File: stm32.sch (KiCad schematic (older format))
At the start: 33 parts, among them P1 USB_OTG, P2 CONN_01X04, U3 STM32F407VETx, U4 USBLC6-4SC6, Y2 25M, Y3 RTC

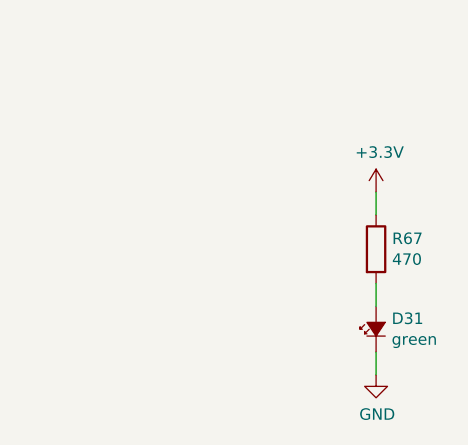
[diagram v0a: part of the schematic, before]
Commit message: eth phy
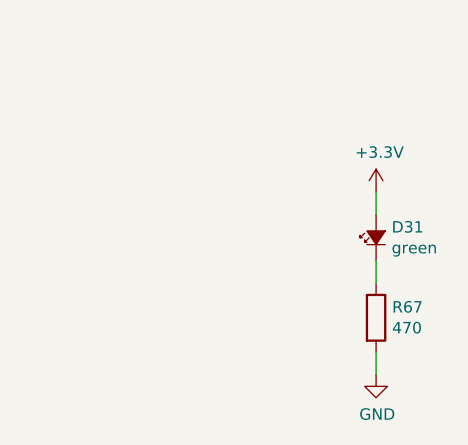
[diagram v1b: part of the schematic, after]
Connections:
- net +3V3: now also D31.2 (A); no longer R67.1
- net GND: now also R67.2; no longer D31.1 (K)
- new net: D31.1 (K), R67.1
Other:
- moved on the sheet: D31, R67
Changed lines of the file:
@@
 L stmbl:Led_Small D31
 U 1 1 5B4CB472
-P 15400 9150
-F 0 "D31" V 15446 9082 50  0000 R CNN
-F 1 "green" V 15355 9082 50  0000 R CNN
-F 2 "stmbl:LED-0805" V 15400 9150 50  0001 C CNN
-F 3 "" V 15400 9150 50  0000 C CNN
-F 4 "LG R971" H 0   0   50  0001 C CNN "Manufacturer No"
-F 5 "Mouser 720-LGR971-KN-1" H 0   0   50  0001 C CNN "Source"
-F 6 "" H 0   0   50  0001 C CNN "Tolerance"
-F 7 "" H 0   0   50  0001 C CNN "Voltage"
-	1    15400 9150
+P 15400 8750
+F 0 "D31" V 15446 8682 50  0000 R CNN
+F 1 "green" V 15355 8682 50  0000 R CNN
+F 2 "stmbl:LED-0805" V 15400 8750 50  0001 C CNN
+F 3 "" V 15400 8750 50  0000 C CNN
+F 4 "LG R971" H 0   -400 50  0001 C CNN "Manufacturer No"
+F 5 "Mouser 720-LGR971-KN-1" H 0   -400 50  0001 C CNN "Source"
+F 6 "" H 0   -400 50  0001 C CNN "Tolerance"
+F 7 "" H 0   -400 50  0001 C CNN "Voltage"
+	1    15400 8750
 	0    -1   -1   0
 $EndComp
@@
 L stmbl:R R67
 U 1 1 5B4CB478
-P 15400 8800
-F 0 "R67" H 15470 8846 50  0000 L CNN
-F 1 "470" H 15470 8755 50  0000 L CNN
-F 2 "stmbl:R_0603" V 15330 8800 50  0001 C CNN
-F 3 "" H 15400 8800 50  0000 C CNN
-F 4 "" H 0   0   50  0001 C CNN "Manufacturer No"
-F 5 "" H 0   0   50  0001 C CNN "Source"
-F 6 "1%" H 0   0   50  0001 C CNN "Tolerance"
-F 7 "" H 0   0   50  0001 C CNN "Voltage"
-	1    15400 8800
+P 15400 9100
+F 0 "R67" H 15470 9146 50  0000 L CNN
+F 1 "470" H 15470 9055 50  0000 L CNN
+F 2 "stmbl:R_0603" V 15330 9100 50  0001 C CNN
+F 3 "" H 15400 9100 50  0000 C CNN
+F 4 "" H 0   300 50  0001 C CNN "Manufacturer No"
+F 5 "" H 0   300 50  0001 C CNN "Source"
+F 6 "1%" H 0   300 50  0001 C CNN "Tolerance"
+F 7 "" H 0   300 50  0001 C CNN "Voltage"
+	1    15400 9100
 	1    0    0    -1
 $EndComp
@@
 Wire Wire Line
 	11250 3600 11400 3600
-Wire Wire Line
-	15400 8950 15400 9050
 Text GLabel 14200 4450 1    60   Input ~ 0
 DC_LINK
@@
 Wire Wire Line
 	8000 3400 8950 3400
+Wire Wire Line
+	15400 8850 15400 8950
 $EndSCHEMATC
